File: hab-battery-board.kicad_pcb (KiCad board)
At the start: 2 copper layers, 30 x 30 mm, 27 parts, among them CN1 XT30PW-M, CN2 S3B-XH-A, CN3 2053380004, J1 Conn_01x06_Pin, Q2 AON7506, U1 BQ296227DSGR, U2 AP63203WU, U3 AP63205WU

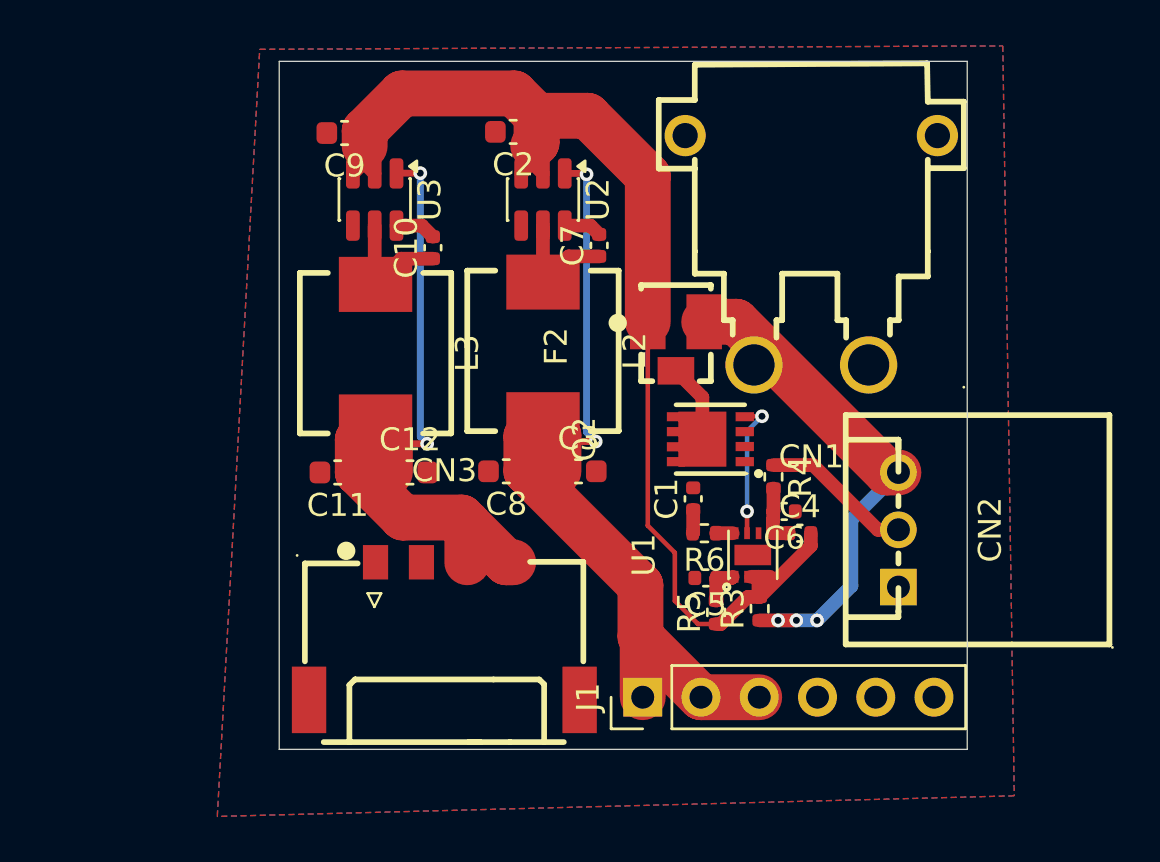
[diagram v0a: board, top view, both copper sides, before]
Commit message: final final
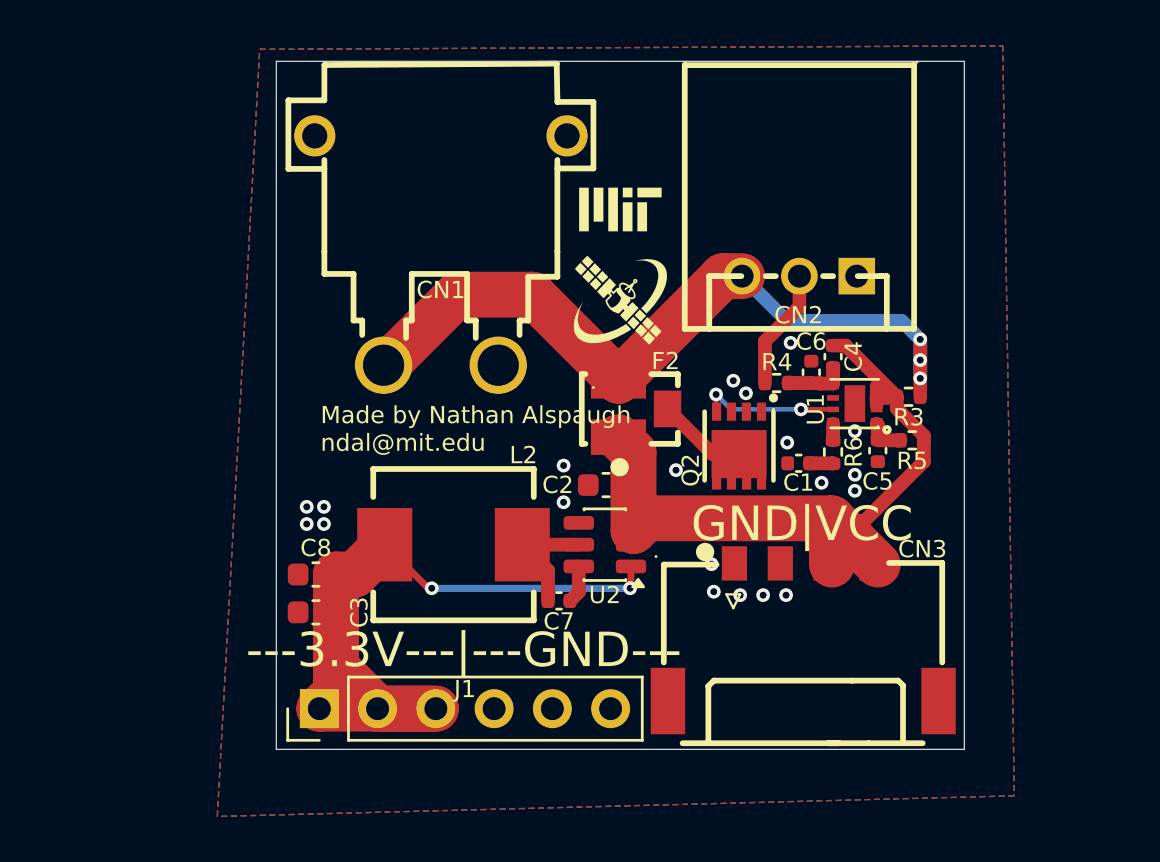
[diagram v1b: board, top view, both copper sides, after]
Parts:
- removed C10: 100nF, Capacitor_SMD:C_0402_1005Metric
- removed C11, C12: 22uF, Capacitor_SMD:C_0603_1608Metric
- removed C9: 10uF, Capacitor_SMD:C_0603_1608Metric
- removed L3: FXL0630-4R7-M, easyeda2kicad:IND-SMD_L7.0-W6.6
- removed U3: AP63205WU, Package_TO_SOT_SMD:TSOT-23-6
- moved CN1 16.2 mm to (150.8, 62.3)
- moved C2 15.9 mm to (158.0, 72.5)
- moved CN3 15.7 mm to (166.6, 79.0)
- moved C7 15.6 mm to (155.9, 77.6), turned to 0 degrees
- moved U2 15.3 mm to (157.9, 75.2), turned to 180 degrees
- moved J1 14.1 mm to (145.5, 82.3)
- moved C3 13.0 mm to (145.3, 78.1), turned to 180 degrees
- moved CN2 11.9 mm to (166.4, 63.4), turned to 0 degrees
- moved R5 11.4 mm to (171.3, 70.6), turned to 180 degrees
- moved R3 11.3 mm to (171.2, 68.7), turned to 180 degrees
- moved C8 9.44 mm to (145.3, 76.5)
- moved C5 9.33 mm to (169.8, 71.0), turned to -90 degrees
- moved L2 9.31 mm to (151.3, 75.2), turned to 180 degrees
- moved U1 7.96 mm to (168.8, 69.0), turned to 180 degrees
- moved C4 7.84 mm to (167.9, 67.0), turned to 90 degrees
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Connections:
- CN3 pad 3: +5V -> VCC
- CN3 pad 4: +5V -> VCC
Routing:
- net +5V: track 30.7 -> 0.00 mm, vias 2 -> 0
- net VCC: track 53.5 -> 31.9 mm
- net /BAT+: track 22.4 -> 33.5 mm
- net +3.3V: track 38.6 -> 31.5 mm
- net Net-(U3-SW): track 5.54 -> 0.00 mm
- net Net-(U3-BST): track 1.79 -> 0.00 mm
- net /BAT_MID: track 6.62 -> 5.28 mm
- net GND: vias 0 -> 20
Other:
- board text added: "---3.3V---|---GND---"
- board text added: "GND|VCC"
- board text added: "Made by Nathan Alspaugh ndal@mit.edu"
